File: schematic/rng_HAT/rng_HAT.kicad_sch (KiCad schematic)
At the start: 32 parts

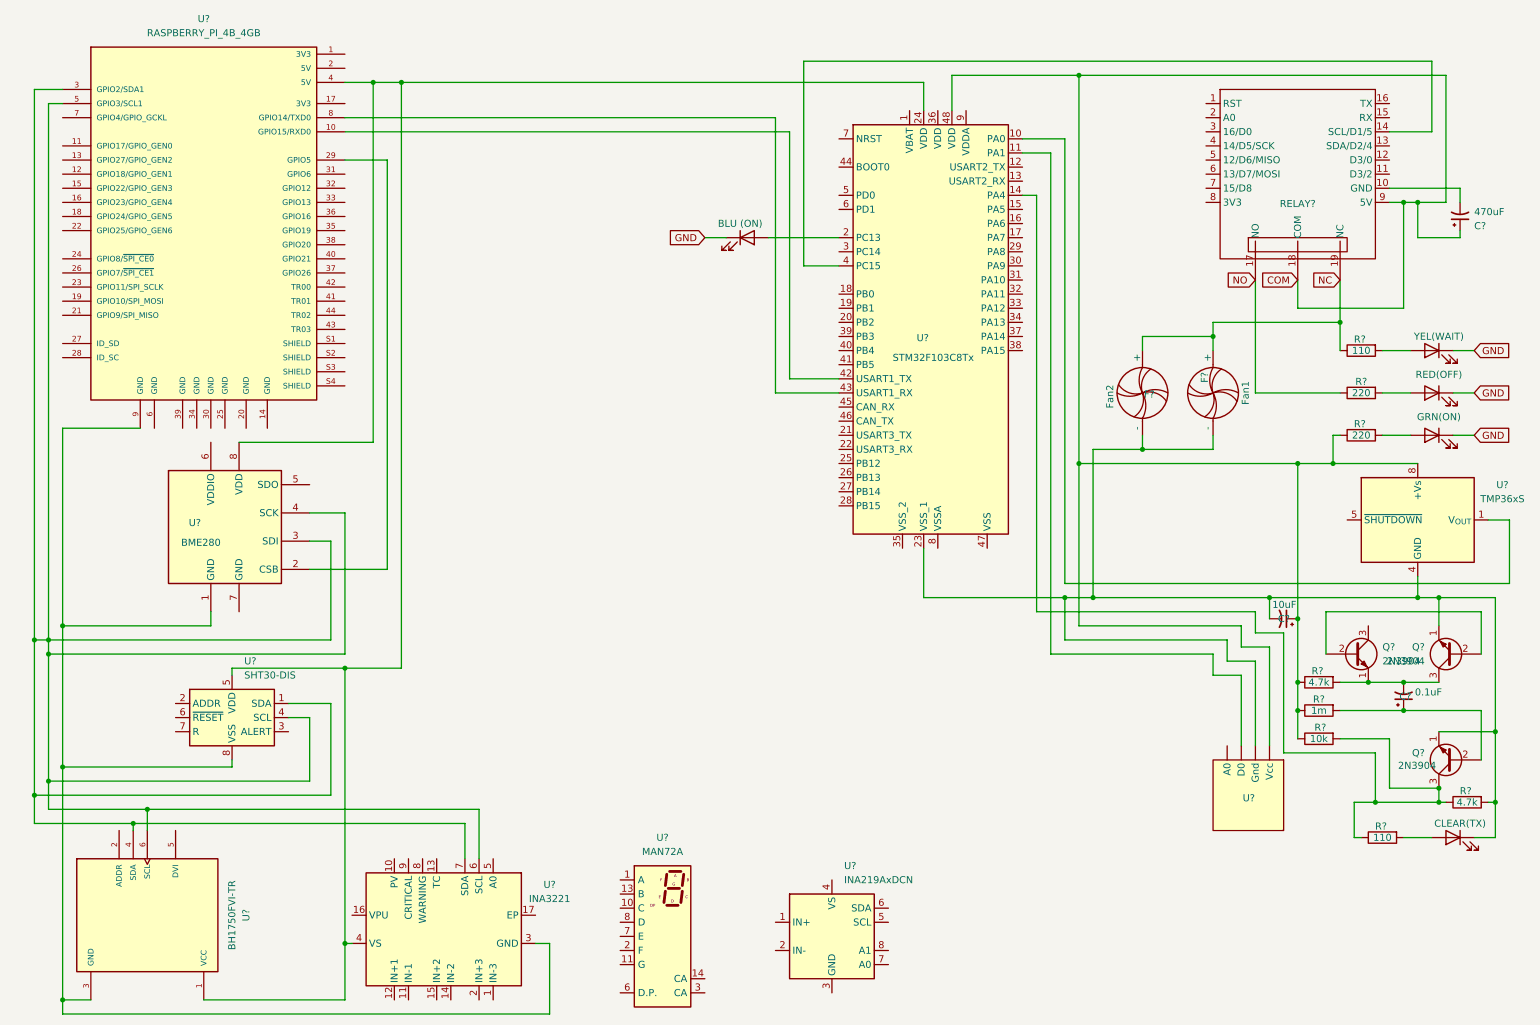
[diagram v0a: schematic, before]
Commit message: updating schematic
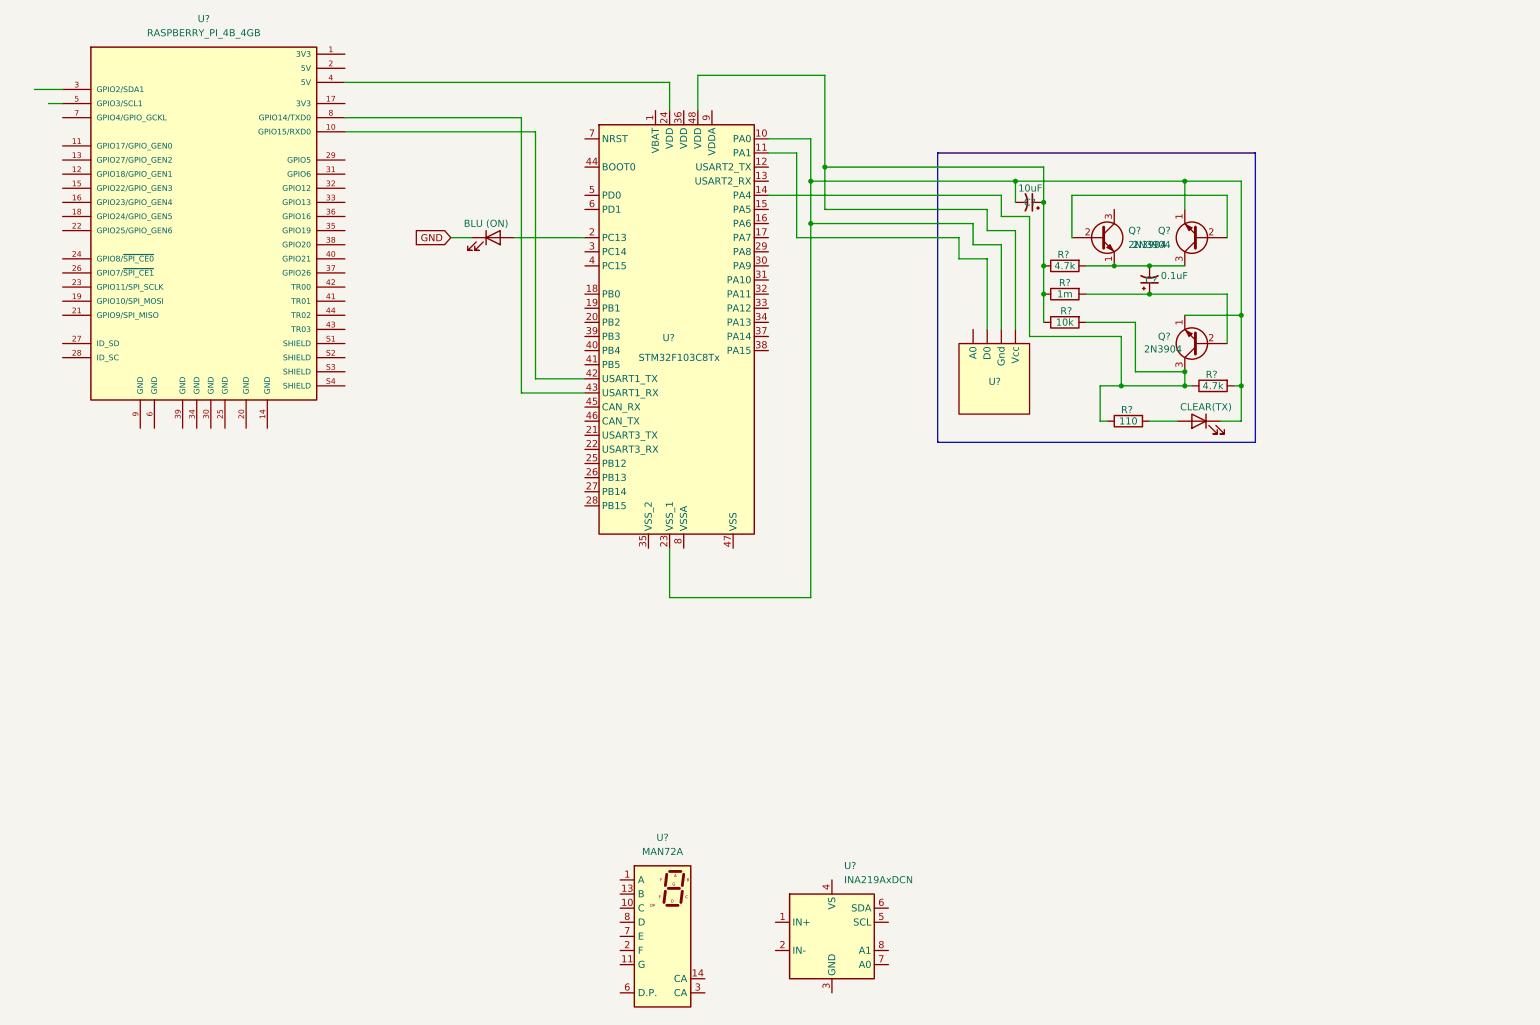
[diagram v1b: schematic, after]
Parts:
- removed C?: 470uF, Capacitor_SMD:CP_Elec_3x5.3, symbol Device:C_Polarized_Small_US
- removed D?: YEL(WAIT), LED_SMD:LED-APA102-2020, symbol Device:LED
- removed D?: GRN(ON), LED_SMD:LED-APA102-2020, symbol Device:LED
- removed D?: RED(OFF), LED_SMD:LED-APA102-2020, symbol Device:LED
- removed F?: Fan1, Connector_PinHeader_2.54mm:PinHeader_1x01_P2.54mm_Horizontal, symbol Motor:Fan_ALT
- removed F?: Fan2, Connector_PinHeader_2.54mm:PinHeader_1x01_P2.54mm_Horizontal, symbol Motor:Fan_ALT
- removed R? (x2): 220, OptoDevice:R_LDR_4.9x4.2mm_P2.54mm_Vertical, symbol Device:R
- removed R?: 110, OptoDevice:R_LDR_4.9x4.2mm_P2.54mm_Vertical, symbol Device:R
- removed RELAY?: ~, symbol my_parts:wemos_relay
- removed U?: INA3221, Package_DFN_QFN:Texas_RGV0016A_VQFN-16-1EP_4x4mm_P0.65mm_EP2.1x2.1mm, symbol Power_Management:INA3221
- removed U?: BME280, Package_LGA:Bosch_LGA-8_2.5x2.5mm_P0.65mm_ClockwisePinNumbering, symbol Sensor:BME280
- removed U?: BH1750FVI-TR, BH1750FVI-TR:XDCR_BH1750FVI-TR, symbol my_parts:BH1750FVI-TR
- removed U?: TMP36xS, Package_SO:SOIC-8_3.9x4.9mm_P1.27mm, symbol Sensor_Temperature:TMP36xS
- removed U?: SHT30-DIS, Sensor_Humidity:Sensirion_DFN-8-1EP_2.5x2.5mm_P0.5mm_EP1.1x1.7mm, symbol Sensor_Humidity:SHT30-DIS
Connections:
- net at C?.2, D?.1 (K), Q?.1 (E)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: now also U?.10 (PA0)
- net at U?.3 (GPIO2/SDA1): no longer U?.5 (GPIO3/SCL1)
- net at U?. (Vcc): now also U?.11 (PA1)
- net COM: no longer names the net of C?.1, R?.1, R?.1, R?.1, U?. (Vcc), U?.48 (VDD)
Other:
- moved on the sheet: C?, Q?, R?, U?

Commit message: updating shematic
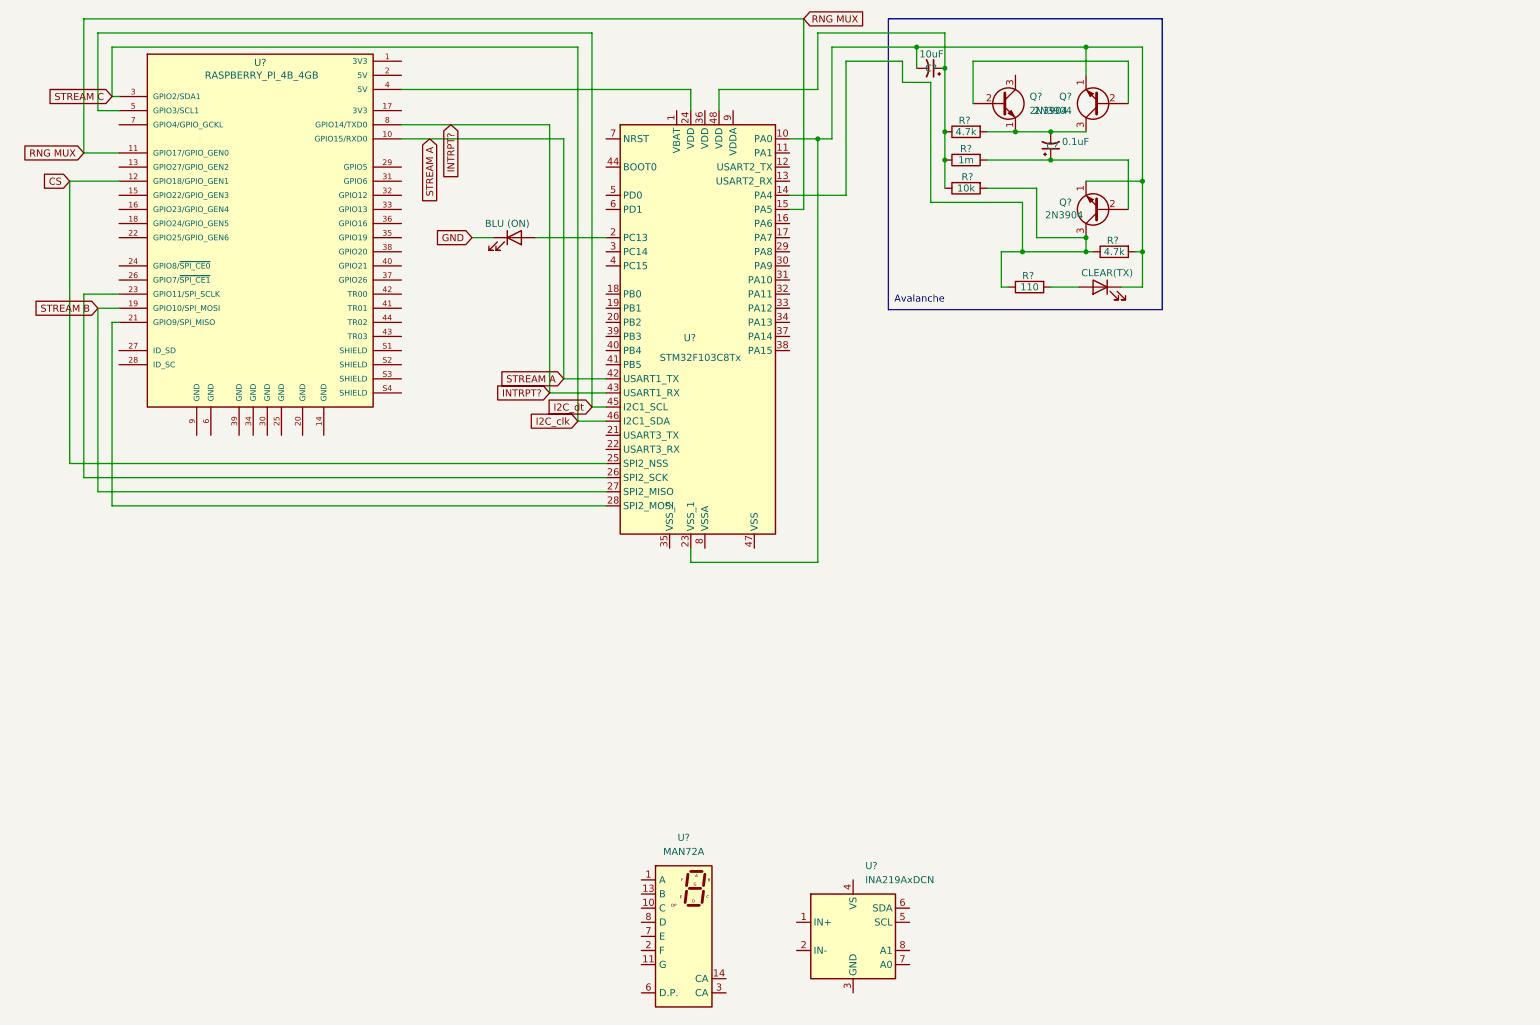
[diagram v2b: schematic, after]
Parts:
- removed U?: ~, symbol my_parts:MQ-6-FF
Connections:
- net STREAM A: now reaches U?.10 (GPIO15/RXD0), U?.42 (PB6)
- net RNG MUX: now reaches U?.11 (GPIO17/GPIO_GEN0)
- net RNG MUX: now also U?.15 (PA5)
- net CS: now reaches U?.12 (GPIO18/GPIO_GEN1)
- net CS: now also U?.25 (PB12)
- net STREAM B: now reaches U?.19 (GPIO10/SPI_MOSI)
- net STREAM B: now also U?.27 (PB14)
- net at U?.21 (GPIO9/SPI_MISO): now also U?.28 (PB15)
- net at U?.23 (GPIO11/SPI_SCLK): now also U?.26 (PB13)
- net I2C_clk: now reaches U?.3 (GPIO2/SDA1)
- net I2C_clk: now also U?.46 (PB9)
- net I2C_dt: now reaches U?.5 (GPIO3/SCL1)
- net I2C_dt: now also U?.45 (PB8)
- net INTRPT?: now reaches U?.43 (PB7), U?.8 (GPIO14/TXD0)
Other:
- note added: "Avalanche"
- moved on the sheet: C?, Q?, R?, U?
